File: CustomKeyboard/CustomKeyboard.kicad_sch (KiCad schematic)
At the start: 178 parts, among them J1 GCT-USB4085, SW1 PEC11H-RotaryEncoderSwitch, U1 ATMEGA32U4-AUR

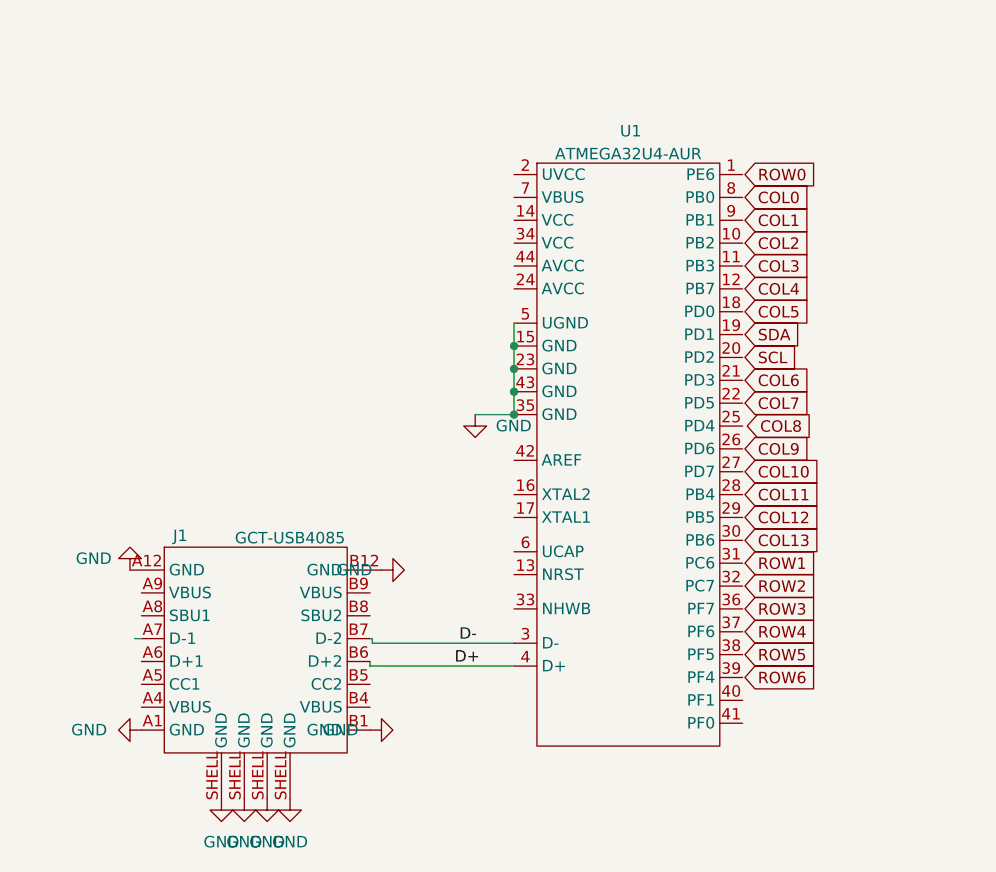
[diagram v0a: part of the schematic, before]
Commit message: stuff
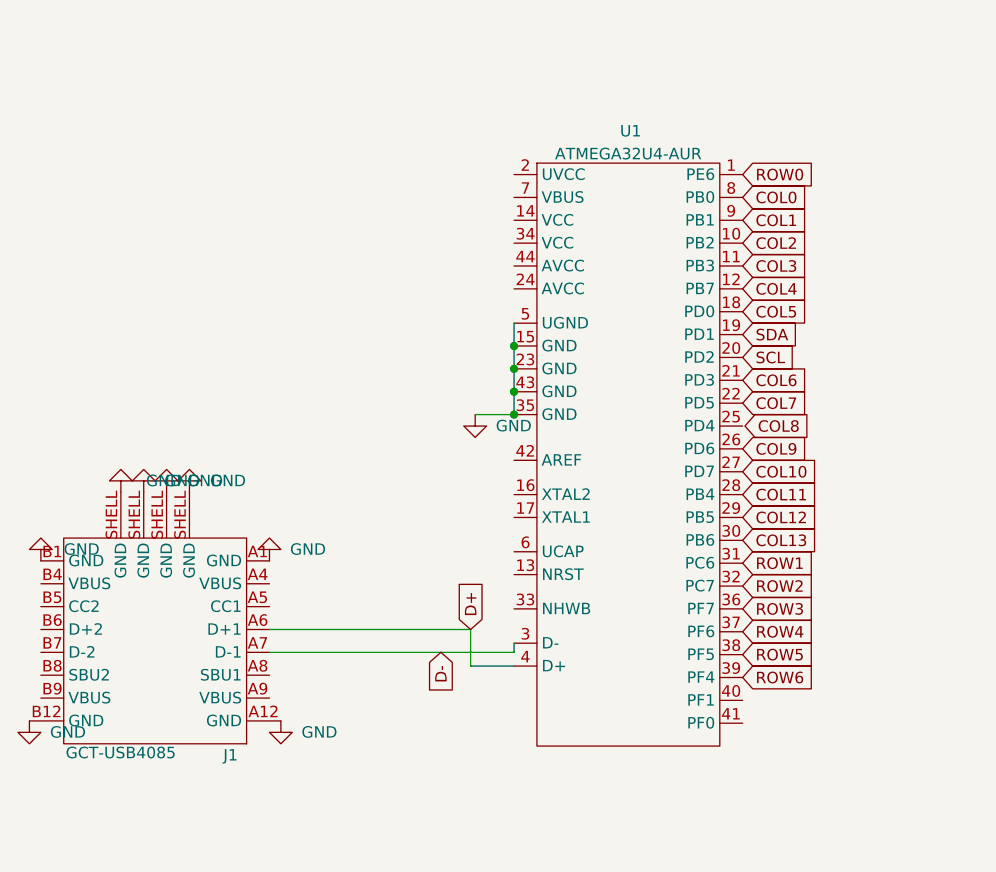
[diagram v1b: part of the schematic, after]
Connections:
- net COL0: now also U1.8 (PB0)
- net COL1: now also U1.9 (PB1)
- net COL10: now also U1.27 (PD7)
- net COL11: now also U1.28 (PB4)
- net COL12: now also U1.29 (PB5)
- net COL13: now also U1.30 (PB6)
- net COL2: now also U1.10 (PB2)
- net COL3: now also U1.11 (PB3)
- net COL4: now also U1.12 (PB7)
- net COL5: now also U1.18 (PD0)
- net COL6: now also U1.21 (PD3)
- net COL7: now also U1.22 (PD5)
- net COL9: now also U1.26 (PD6)
- net D+: now also J1.A6 (D+1); no longer J1.B6 (D+2)
- net D-: now also J1.A7 (D-1); no longer J1.B7 (D-2)
- net ROW0: now also U1.1 (PE6)
- net ROW1: now also U1.31 (PC6)
- net ROW2: now also U1.32 (PC7)
- net ROW3: now also U1.36 (PF7)
- net ROW4: now also U1.37 (PF6)
- net ROW5: now also U1.38 (PF5)
- net ROW6: now also U1.39 (PF4)
- net SCL: now also U1.20 (PD2)
- net SDA: now also U1.19 (PD1)
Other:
- moved on the sheet: J1
